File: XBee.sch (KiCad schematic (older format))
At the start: 3 parts, among them U2 XBP24-AWI-001

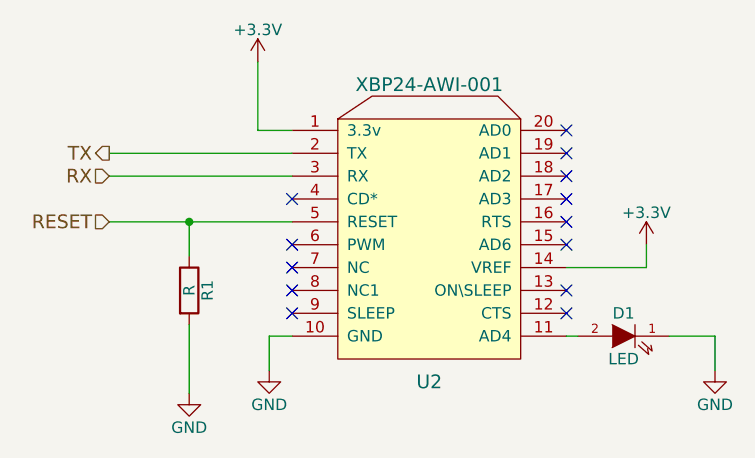
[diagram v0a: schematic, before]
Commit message: Ruteo. Correciones. Cambio de footprint del switch.
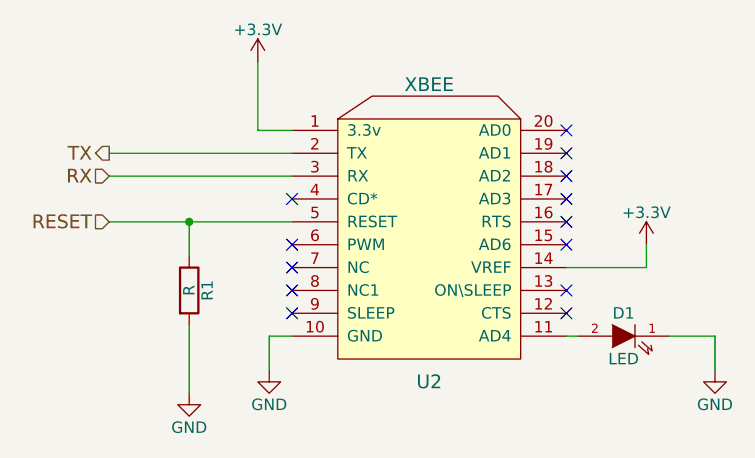
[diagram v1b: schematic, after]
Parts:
- U2: value XBP24-AWI-001 -> XBEE; footprint XBee:XBee-pro -> footprints:XBee-pro; Desc (none) -> XBee-PRO S1 802.15.4 extended-range module w/ wire antenna; Manf# (none) -> XBP24-AWI-001
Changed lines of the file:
@@
 encoding utf-8
 Sheet 3 4
-Title ""
-Date ""
-Rev ""
+Title "Poncho Misión SAEv2 - Módulo XBee"
+Date "2016-12-14"
+Rev "1.0"
 Comp ""
-Comment1 ""
-Comment2 ""
+Comment1 "Autores: Julián Iglesias / Elli Carlos"
+Comment2 "Licencia: BSD"
 Comment3 ""
 Comment4 ""
@@
 $Comp
 L XBEE U2
-U 1 1 58325202
+U 1 1 5851DFE8
 P 3900 3200
 F 0 "U2" H 3900 2650 60  0000 C CNN
-F 1 "XBP24-AWI-001" H 3900 3950 60  0000 C CNN
-F 2 "XBee:XBee-pro" H 3900 3200 60  0001 C CNN
+F 1 "XBEE" H 3900 3950 60  0000 C CNN
+F 2 "footprints:XBee-pro" H 3900 3200 60  0001 C CNN
 F 3 "https://www.digi.com/pdf/ds_xbeemultipointmodules.pdf" H 3900 3200 60  0001 C CNN
-F 4 "DIGI" H 3900 3200 60  0001 C CNN "Manf"
-F 5 "XB24-AWI-001
-" H 3900 3200 60  0001 C CNN "Manf#"
-F 6 "XB24-AWI-001-ND
+F 4 "XBee-PRO S1 802.15.4 extended-range module w/ wire antenna" H 3900 3200 60  0001 C CNN "Desc"
+F 5 "DIGI" H 3900 3200 60  0001 C CNN "Manf"
+F 6 "XBP24-AWI-001" H 3900 3200 60  0001 C CNN "Manf#"
+F 7 "XBP24-AWI-001-ND
 " H 3900 3200 60  0001 C CNN "Digikey#"
-F 7 "888-XB24-AWI-001
+F 8 "888-XBP24-AWI-001
 " H 3900 3200 60  0001 C CNN "Mouser#"
 	1    3900 3200

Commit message: Corrección de errores in progress...
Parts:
- U2: Desc XBee-PRO S1 802.15.4 extended-range module w/ wire antenna -> XBee Pro Series1 Wire antenna; Digikey# (none) -> XBP24-AWI-001-ND; Mouser# (none) -> 888-XBP24-AWI-001
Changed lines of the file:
@@
 EESchema Schematic File Version 2
-LIBS:Mision_SAE-rescue
 LIBS:power
-LIBS:device
-LIBS:conn
-LIBS:mpu-6050
-LIBS:power1
-LIBS:xbee
-LIBS:basico
-LIBS:GY-65
-LIBS:GY-521
 LIBS:Mision_SAE-cache
 EELAYER 25 0
@@
 encoding utf-8
 Sheet 3 4
-Title "Poncho Misión SAEv2 - Módulo XBee"
-Date "2016-12-14"
+Title "Poncho Misión SAEv2 - Esquemático jerárquico"
+Date "2016-12-21"
 Rev "1.0"
 Comp ""
-Comment1 "Autores: Julián Iglesias / Elli Carlos"
-Comment2 "Licencia: BSD"
-Comment3 ""
+Comment1 "Autores: Julián Iglesias / Elli Carlos."
+Comment2 "Revisor: Matías Marando"
+Comment3 "Licencia: BSD"
 Comment4 ""
 $EndDescr
@@
 $EndComp
 $Comp
-L GND #PWR013
+L GND #PWR011
 U 1 1 583259FC
 P 5150 3700
-F 0 "#PWR013" H 5150 3450 50  0001 C CNN
+F 0 "#PWR011" H 5150 3450 50  0001 C CNN
 F 1 "GND" H 5150 3550 50  0000 C CNN
 F 2 "" H 5150 3700 50  0000 C CNN
@@
 $EndComp
 $Comp
-L GND #PWR014
+L GND #PWR012
 U 1 1 58325A17
 P 3200 3700
-F 0 "#PWR014" H 3200 3450 50  0001 C CNN
+F 0 "#PWR012" H 3200 3450 50  0001 C CNN
 F 1 "GND" H 3200 3550 50  0000 C CNN
 F 2 "" H 3200 3700 50  0000 C CNN
@@
 $EndComp
 $Comp
-L GND #PWR015
+L GND #PWR013
 U 1 1 58325A2B
 P 2850 3800
-F 0 "#PWR015" H 2850 3550 50  0001 C CNN
+F 0 "#PWR013" H 2850 3550 50  0001 C CNN
 F 1 "GND" H 2850 3650 50  0000 C CNN
 F 2 "" H 2850 3800 50  0000 C CNN
@@
 $EndComp
 $Comp
-L +3.3V #PWR016
+L +3.3V #PWR014
 U 1 1 58325A3E
 P 3150 2350
-F 0 "#PWR016" H 3150 2200 50  0001 C CNN
+F 0 "#PWR014" H 3150 2200 50  0001 C CNN
 F 1 "+3.3V" H 3150 2490 50  0000 C CNN
 F 2 "" H 3150 2350 50  0000 C CNN
@@
 NoConn ~ 4500 3150
 $Comp
-L +3.3V #PWR017
+L +3.3V #PWR015
 U 1 1 58325B5C
 P 4850 3150
-F 0 "#PWR017" H 4850 3000 50  0001 C CNN
+F 0 "#PWR015" H 4850 3000 50  0001 C CNN
 F 1 "+3.3V" H 4850 3290 50  0000 C CNN
 F 2 "" H 4850 3150 50  0000 C CNN
@@
 $Comp
 L XBEE U2
-U 1 1 5851DFE8
+U 1 1 585B02E9
 P 3900 3200
 F 0 "U2" H 3900 2650 60  0000 C CNN
@@
 F 2 "footprints:XBee-pro" H 3900 3200 60  0001 C CNN
 F 3 "https://www.digi.com/pdf/ds_xbeemultipointmodules.pdf" H 3900 3200 60  0001 C CNN
-F 4 "XBee-PRO S1 802.15.4 extended-range module w/ wire antenna" H 3900 3200 60  0001 C CNN "Desc"
+F 4 "XBee Pro Series1 Wire antenna" H 3900 3200 60  0001 C CNN "Desc"
 F 5 "DIGI" H 3900 3200 60  0001 C CNN "Manf"
 F 6 "XBP24-AWI-001" H 3900 3200 60  0001 C CNN "Manf#"
-F 7 "XBP24-AWI-001-ND
-" H 3900 3200 60  0001 C CNN "Digikey#"
-F 8 "888-XBP24-AWI-001
-" H 3900 3200 60  0001 C CNN "Mouser#"
+F 7 "XBP24-AWI-001-ND" H 3900 3200 60  0001 C CNN "Digikey#"
+F 8 "888-XBP24-AWI-001" H 3900 3200 60  0001 C CNN "Mouser#"
 	1    3900 3200
 	1    0    0    -1
